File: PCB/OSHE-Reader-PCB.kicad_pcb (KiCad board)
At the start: 2 copper layers, 80 x 100 mm, 74 parts, among them J1 UART, J2 112L-TDA0, J3 JTAG, J5 boot_select, Q1 Si1308EDL, Q2 BSS138, Q3 BSS138, U1 74LVC1G04, U2 TPS923610DRLR, U3 TLV75533PDBV, U4 ESP32-S3-WROOM-1

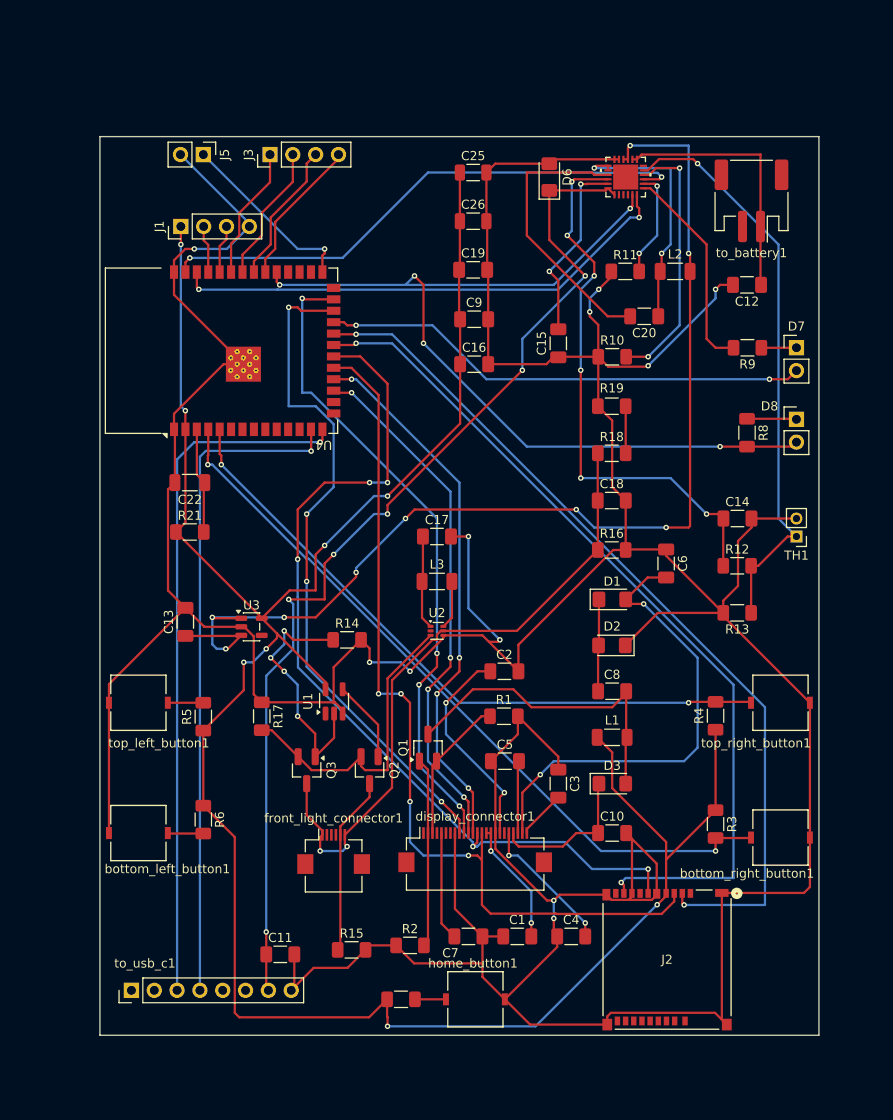
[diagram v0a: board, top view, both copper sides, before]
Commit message: pcb
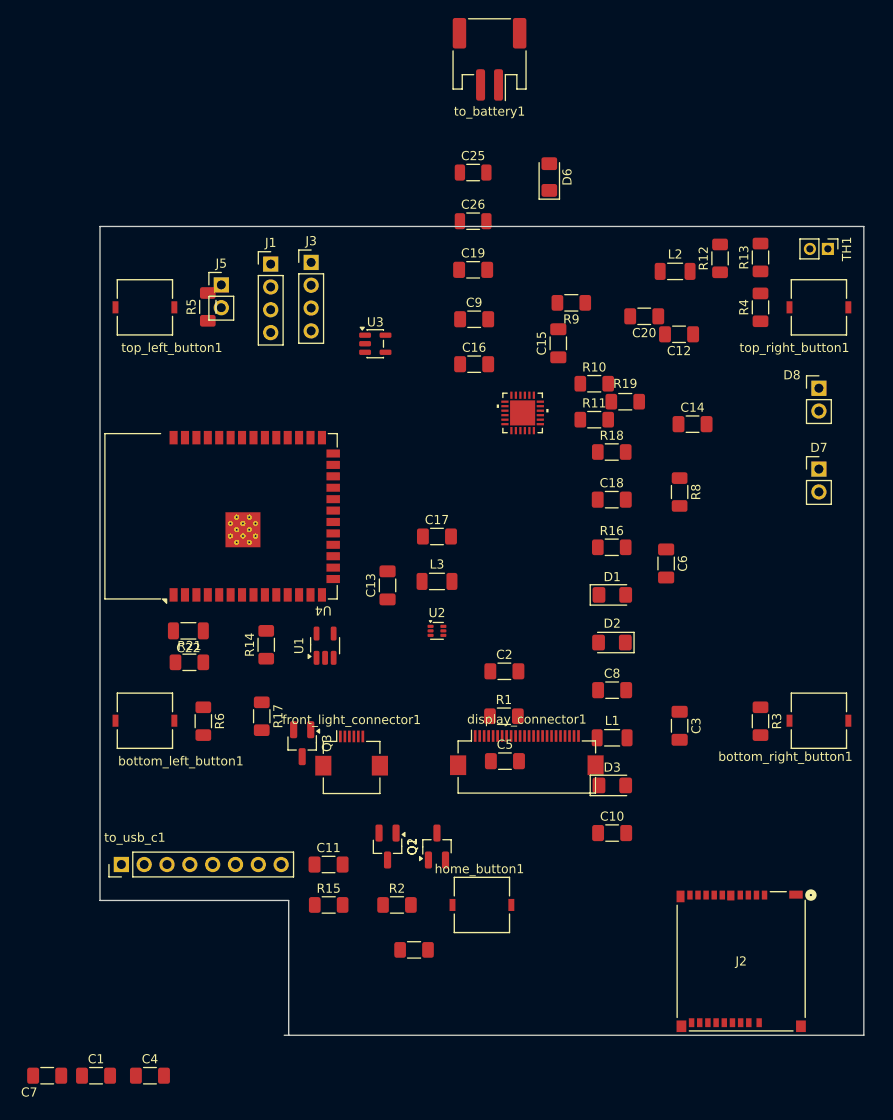
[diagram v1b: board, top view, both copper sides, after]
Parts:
- moved C1 49.4 mm to (113.1, 153.0)
- moved C4 49.4 mm to (119.1, 153.0)
- moved C7 49.4 mm to (107.6, 153.0)
- moved R4 45.7 mm to (187.0, 67.5)
- moved R5 45.6 mm to (125.5, 67.5)
- moved top_right_button1 44.2 mm to (193.5, 67.5)
- moved top_left_button1 44.0 mm to (118.5, 67.5), turned to 0 degrees
- moved R13 39.6 mm to (187.0, 62.0), turned to 90 degrees
- moved U3 34.4 mm to (144.1, 71.5)
- moved R12 34.3 mm to (182.5, 62.0), turned to 90 degrees
- moved to_battery1 33.1 mm to (156.8, 39.9)
- moved TH1 32.2 mm to (194.5, 61.0), turned to -90 degrees
- moved battery_manager1 28.6 mm to (160.5, 79.2)
- moved C13 22.9 mm to (145.5, 98.4)
- moved R9 20.2 mm to (165.9, 67.0)
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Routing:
- net GND: track 551.1 -> 0.00 mm, vias 11 -> 0
- net +3V3: track 263.7 -> 0.00 mm, vias 8 -> 0
- net /Battery Charger/SYS: track 127.2 -> 0.00 mm, vias 9 -> 0
- net /VBUS: track 116.8 -> 0.00 mm, vias 6 -> 0
- net /STAT: track 101.5 -> 0.00 mm, vias 5 -> 0
- net /SCL: track 100.4 -> 0.00 mm, vias 5 -> 0
- net /COPI: track 99.0 -> 0.00 mm, vias 4 -> 0
- net /SD_CS: track 97.6 -> 0.00 mm, vias 2 -> 0
- net /CIPO: track 95.9 -> 0.00 mm, vias 2 -> 0
- net /BR_button: track 83.7 -> 0.00 mm, vias 2 -> 0
- net /D+: track 77.3 -> 0.00 mm, vias 1 -> 0
- net /BUSY: track 75.8 -> 0.00 mm, vias 4 -> 0
- net /D-: track 74.5 -> 0.00 mm, vias 1 -> 0
- net /TR_button: track 74.0 -> 0.00 mm, vias 2 -> 0
- net /RES_SCR: track 72.7 -> 0.00 mm, vias 4 -> 0
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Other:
- board size 80 x 100 mm -> 85 x 90 mm
- board text added: "screen"
